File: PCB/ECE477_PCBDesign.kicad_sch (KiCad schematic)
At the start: 0 parts

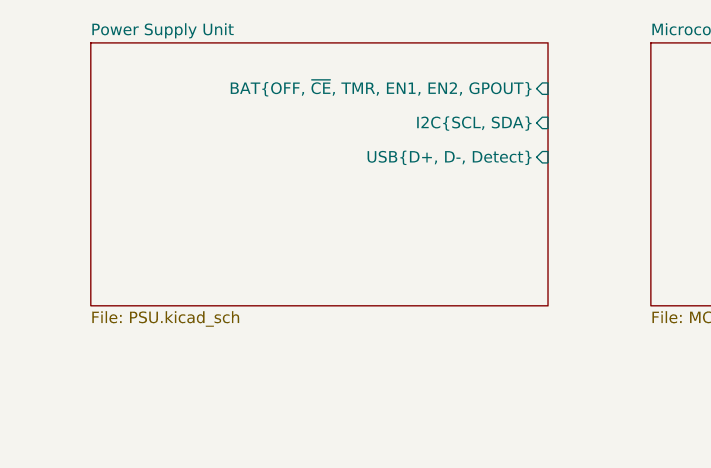
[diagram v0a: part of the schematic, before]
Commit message: PCB update - Minh
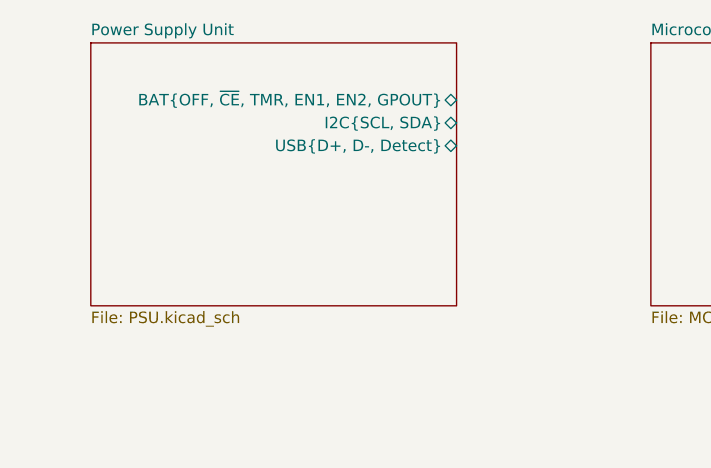
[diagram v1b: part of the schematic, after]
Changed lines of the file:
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@@
     )
   )
-  (sheet (at 121.92 110.49) (size 50.8 29.21) (fields_autoplaced)
+  (sheet (at 121.92 110.49) (size 40.64 29.21) (fields_autoplaced)
     (stroke (width 0.1524) (type solid))
     (fill (color 0 0 0 0.0000))
@@
       (effects (font (size 1.27 1.27)) (justify left top))
     )
-    (pin "USB{D+, D-, Detect}" input (at 172.72 123.19 0)
+    (pin "BAT{OFF, ~{CE}, TMR, EN1, EN2, GPOUT}" bidirectional (at 162.56 116.84 0)
       (effects (font (size 1.27 1.27)) (justify right))
     )
-    (pin "I2C{SCL, SDA}" input (at 172.72 119.38 0)
+    (pin "I2C{SCL, SDA}" bidirectional (at 162.56 119.38 0)
       (effects (font (size 1.27 1.27)) (justify right))
     )
-    (pin "BAT{OFF, ~{CE}, TMR, EN1, EN2, GPOUT}" input (at 172.72 115.57 0)
+    (pin "USB{D+, D-, Detect}" bidirectional (at 162.56 121.92 0)
       (effects (font (size 1.27 1.27)) (justify right))
     )

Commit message: Revert "PCB update - Minh"
This reverts commit 0608947e49f54a64abc006b190e3b029bac40ad1.
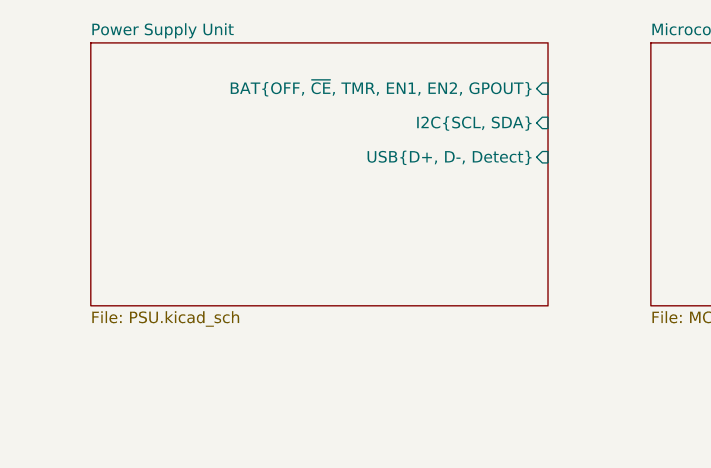
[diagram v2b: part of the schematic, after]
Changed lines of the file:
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@@
     )
   )
-  (sheet (at 121.92 110.49) (size 40.64 29.21) (fields_autoplaced)
+  (sheet (at 121.92 110.49) (size 50.8 29.21) (fields_autoplaced)
     (stroke (width 0.1524) (type solid))
     (fill (color 0 0 0 0.0000))
@@
       (effects (font (size 1.27 1.27)) (justify left top))
     )
-    (pin "BAT{OFF, ~{CE}, TMR, EN1, EN2, GPOUT}" bidirectional (at 162.56 116.84 0)
+    (pin "USB{D+, D-, Detect}" input (at 172.72 123.19 0)
       (effects (font (size 1.27 1.27)) (justify right))
     )
-    (pin "I2C{SCL, SDA}" bidirectional (at 162.56 119.38 0)
+    (pin "I2C{SCL, SDA}" input (at 172.72 119.38 0)
       (effects (font (size 1.27 1.27)) (justify right))
     )
-    (pin "USB{D+, D-, Detect}" bidirectional (at 162.56 121.92 0)
+    (pin "BAT{OFF, ~{CE}, TMR, EN1, EN2, GPOUT}" input (at 172.72 115.57 0)
       (effects (font (size 1.27 1.27)) (justify right))
     )
